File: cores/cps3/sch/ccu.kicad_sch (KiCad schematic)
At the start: 2 parts, among them J13 DL-2829-CCU

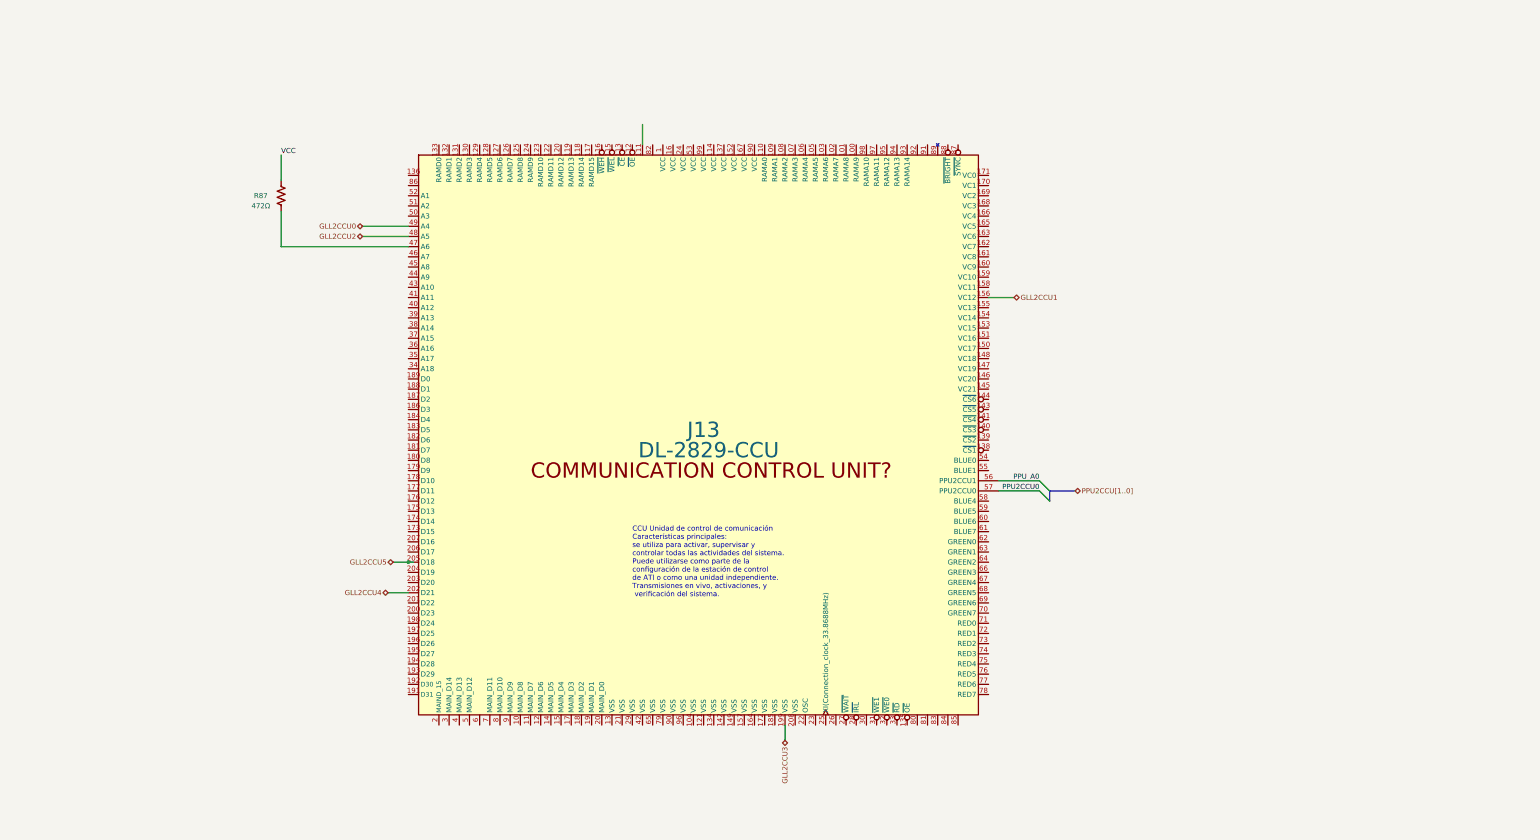
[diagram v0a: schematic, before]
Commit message: wip_ccu_gll2_cassette
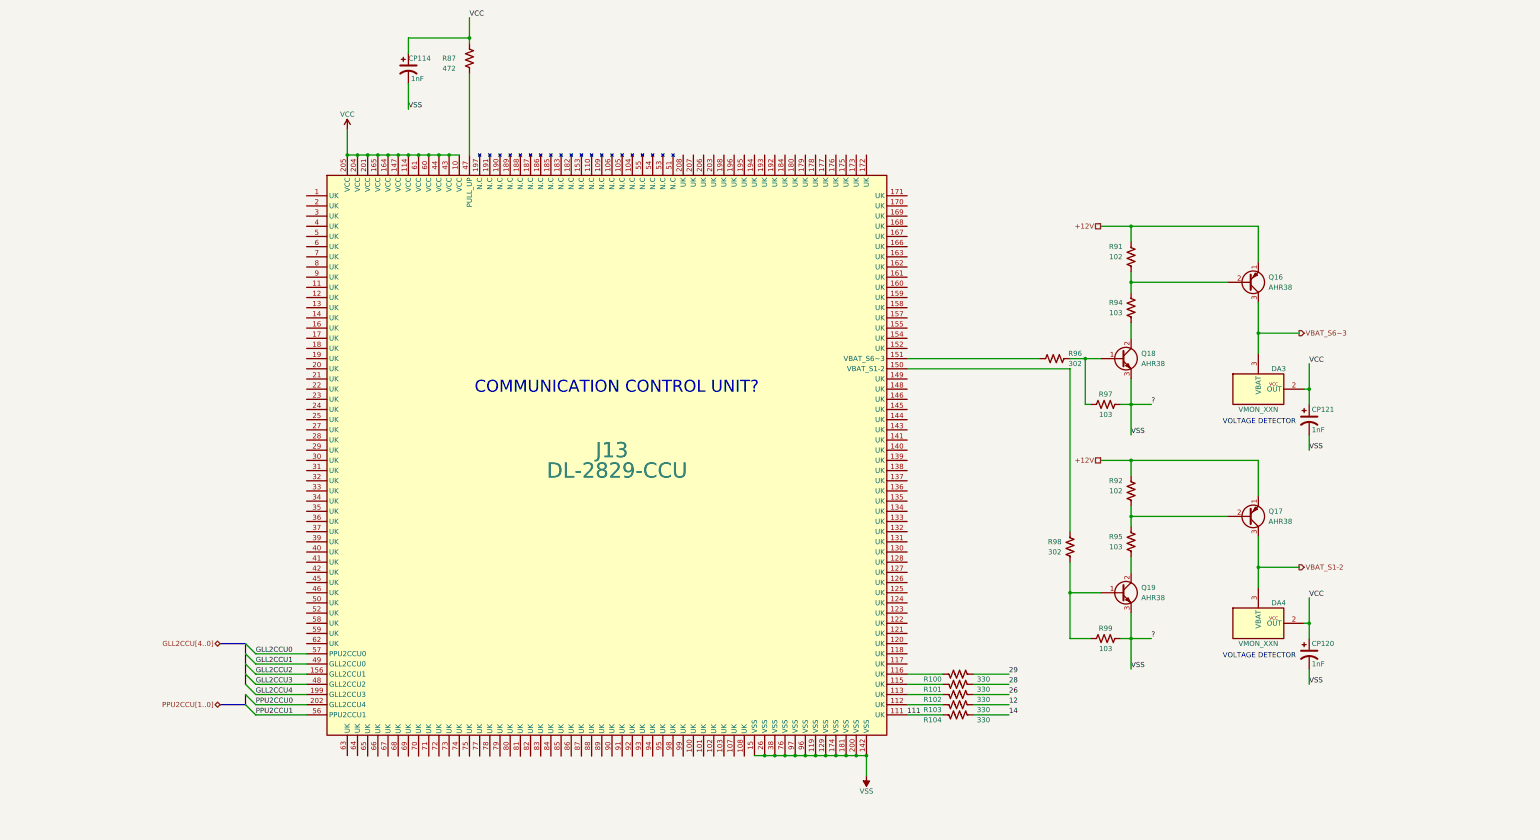
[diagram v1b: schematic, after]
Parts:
- added CP114, CP120, CP121: 1nF, symbol Device:C_Polarized_US
- added DA3, DA4: VMON_XXN, symbol arcade:VMON_XXN
- added Q16, Q17: AHR38, symbol Device:Q_PNP_EBC
- added Q18, Q19: AHR38, symbol Device:Q_NPN_BCE
- added R100, R101, R102, R103, R104: 330, symbol Device:R_US
- added R91, R92: 102, symbol Device:R_US
- added R94, R95, R97, R99: 103, symbol Device:R_US
- added R96, R98: 302, symbol Device:R_US
- R87: value 472Ω -> 472
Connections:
- net GLL2CCU5 is gone; now on net VCC: J13.205 (VCC)
- net GLL2CCU0: now also J13.57 (PPU2CCU0); no longer J13.49 (A4)
- net GLL2CCU1: now also J13.49 (GLL2CCU0); no longer J13.156 (VC12)
- net GLL2CCU2: now also J13.156 (GLL2CCU1); no longer J13.48 (A5)
- net GLL2CCU3: now also J13.48 (GLL2CCU2); no longer J13.199 (VSS)
- net GLL2CCU4: now also J13.199 (GLL2CCU3); no longer J13.202 (D21)
- net PPU2CCU0: now also J13.202 (GLL2CCU4); no longer J13.57 (PPU2CCU0)
- net VCC: now also J13.10 (VCC), J13.114 (VCC), J13.147 (VCC), J13.164 (VCC), J13.165 (VCC), J13.201 (VCC), J13.204 (VCC), J13.43 (VCC), J13.44 (VCC), J13.60 (VCC), J13.61 (VCC), CP114.1, CP120.1, CP121.1, DA3.2 (OUT), DA4.2 (OUT)
- net 111: now reaches J13.111 (UK)
- net 111: now also R104.1
- net at J13.112 (UK): now also R103.1
- net at J13.113 (UK): now also R102.1
- net at J13.115 (UK): now also R101.1
- net at J13.116 (UK): now also R100.1
- net VSS: now reaches J13.119 (VSS)
- net VSS: now also J13.129 (VSS), J13.142 (VSS), J13.15 (VSS), J13.174 (VSS), J13.181 (VSS), J13.200 (VSS), J13.26 (VSS), J13.38 (VSS), J13.76 (VSS), J13.96 (VSS), J13.97 (VSS), CP114.2, CP120.2, CP121.2, DA3.1 (VSS), DA4.1 (VSS), Q18.3 (E), Q19.3 (E), R97.2, R99.2
- net at J13.150 (VBAT_S1-2): now also R98.2
- net at J13.151 (VBAT_S6~3): now also R96.1
- net PPU_A0 renamed PPU2CCU1
- new net: Q18.1 (B), R96.2, R97.1
- new net: Q19.1 (B), R98.1, R99.1
- new net: Q19.2 (C), R95.2
- new net: Q18.2 (C), R94.2
- new net: Q16.2 (B), R91.1, R94.1
- new net: Q17.2 (B), R92.1, R95.1
- new net +12V: Q16.1 (E), Q17.1 (E), R91.2, R92.2
- new net 12: R103.2
- new net 14: R104.2
- new net 26: R102.2
- new net 28: R101.2
- new net 29: R100.2
- new net VBAT_S1-2: DA4.3 (VBAT), Q17.3 (C)
- new net VBAT_S6~3: DA3.3 (VBAT), Q16.3 (C)
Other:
- note added: "COMMUNICATION CONTROL UNIT?"
- note added: "VOLTAGE DETECTOR"
- note removed: "CCU Unidad de control de comunicación Características principales: se utiliza para activar, supervisar y controlar todas las actividades del sistema. Puede utilizarse como parte de la conﬁguración de la estación de control de ATI o como una unidad independiente. Transmisiones en vivo, activaciones, y veriﬁcación del sistema."
- moved on the sheet: R87

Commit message: wip_ccu_cassette
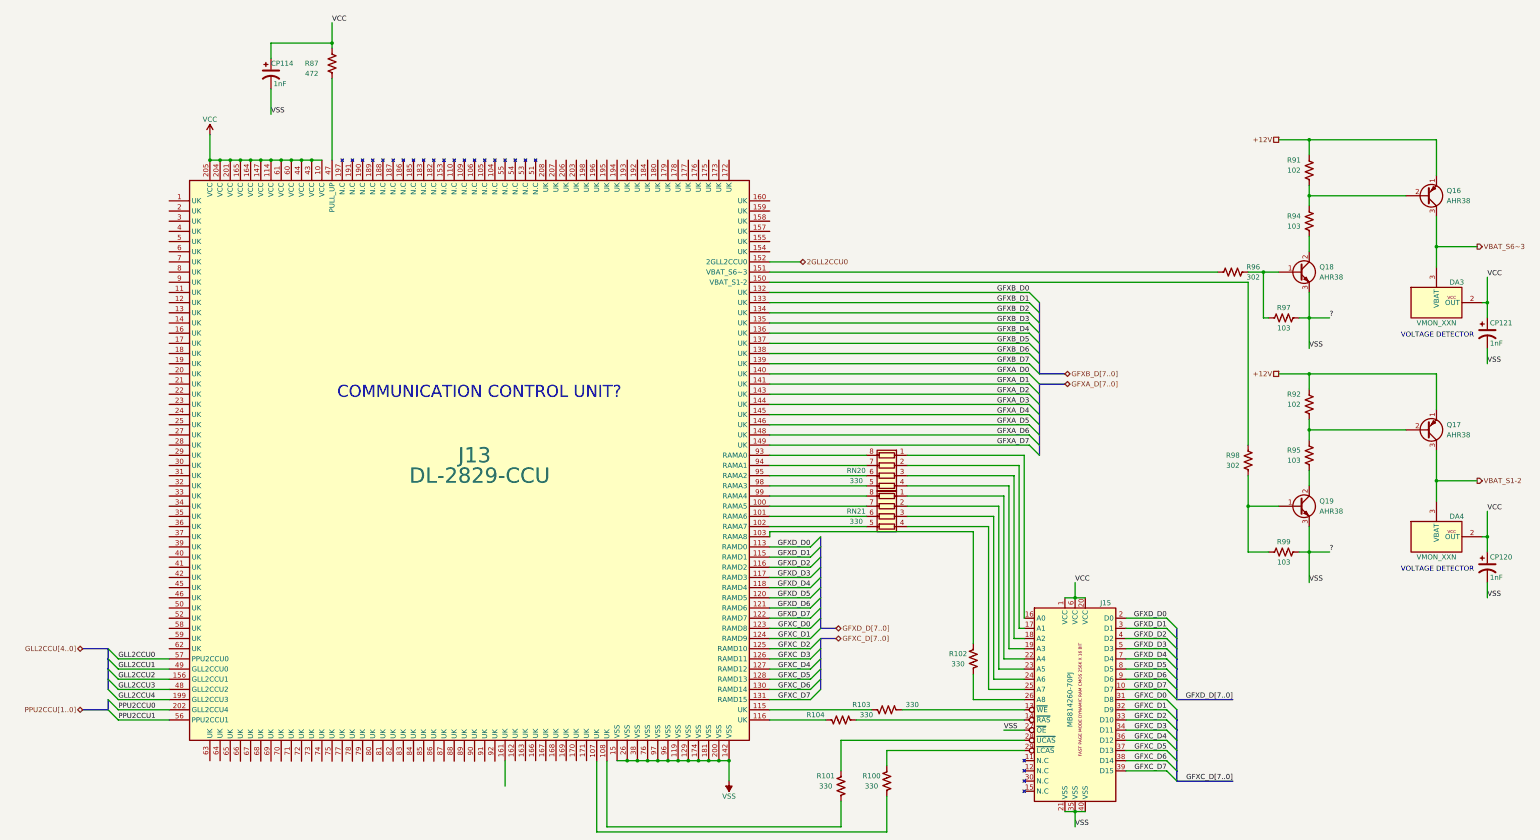
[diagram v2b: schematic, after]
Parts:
- added J15: MB814260-70PJ, symbol fujitsu:MB814260-70PJ
- added RN20, RN21: 330, symbol Device:R_Pack04
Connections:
- net 28 is gone; now on an unnamed net: R101.2
- net 29 is gone; now on an unnamed net: R100.2
- net VCC: now also J15.1 (VCC), J15.20 (VCC), J15.6 (VCC)
- net VSS: now also J15.21 (VSS), J15.27 (~{OE}), J15.35 (VSS), J15.40 (VSS)
- net at R102.1: now also J13.103 (RAMA8); no longer J13.113 (UK)
- net at R100.1: now also J15.29 (~{LCAS}); no longer J13.116 (UK)
- net at J13.100 (RAMA5): now also RN21.7 (R2.2)
- net at J13.101 (RAMA6): now also RN21.6 (R3.2)
- net at J13.102 (RAMA7): now also RN21.5 (R4.2)
- net at R103.1: now also J13.115 (UK); no longer J13.112 (UK)
- net at R101.1: now also J15.28 (~{UCAS}); no longer J13.115 (UK)
- net GFXD_D3: now reaches J13.117 (RAMD3)
- net GFXD_D3: now also J15.5 (D3)
- net GFXD_D4: now reaches J13.118 (RAMD4)
- net GFXD_D4: now also J15.7 (D4)
- net GFXD_D5: now reaches J13.120 (RAMD5)
- net GFXD_D5: now also J15.8 (D5)
- net GFXD_D6: now reaches J13.121 (RAMD6)
- net GFXD_D6: now also J15.9 (D6)
- net GFXD_D7: now reaches J13.122 (RAMD7)
- net GFXD_D7: now also J15.10 (D7)
- net GFXC_D0: now reaches J13.123 (RAMD8)
- net GFXC_D0: now also J15.31 (D8)
- net GFXC_D1: now reaches J13.124 (RAMD9)
- net GFXC_D1: now also J15.32 (D9)
- net GFXC_D2: now reaches J13.125 (RAMD10)
- net GFXC_D2: now also J15.33 (D10)
- net GFXC_D3: now reaches J13.126 (RAMD11)
- net GFXC_D3: now also J15.34 (D11)
- net GFXC_D4: now reaches J13.127 (RAMD12)
- net GFXC_D4: now also J15.36 (D12)
- net GFXC_D5: now reaches J13.128 (RAMD13)
- net GFXC_D5: now also J15.37 (D13)
- net GFXC_D6: now reaches J13.130 (RAMD14)
- net GFXC_D6: now also J15.38 (D14)
- net GFXC_D7: now reaches J13.131 (RAMD15)
- net GFXC_D7: now also J15.39 (D15)
- net GFXB_D0: now reaches J13.132 (UK)
- net GFXB_D1: now reaches J13.133 (UK)
- net GFXB_D2: now reaches J13.134 (UK)
- net GFXB_D3: now reaches J13.135 (UK)
- net GFXB_D4: now reaches J13.136 (UK)
- net GFXB_D5: now reaches J13.137 (UK)
- net GFXB_D6: now reaches J13.138 (UK)
- net GFXB_D7: now reaches J13.139 (UK)
- net GFXA_D0: now reaches J13.140 (UK)
- net GFXA_D1: now reaches J13.141 (UK)
- net GFXA_D2: now reaches J13.143 (UK)
- net GFXA_D3: now reaches J13.144 (UK)
- net GFXA_D4: now reaches J13.145 (UK)
- net GFXA_D5: now reaches J13.146 (UK)
- net GFXA_D6: now reaches J13.148 (UK)
- net GFXA_D7: now reaches J13.149 (UK)
- net 2GLL2CCU0: now reaches J13.152 (2GLL2CCU0)
- net at J13.93 (RAMA0): now also RN20.8 (R1.2)
- net at J13.94 (RAMA1): now also RN20.7 (R2.2)
- net at J13.95 (RAMA2): now also RN20.6 (R3.2)
- net at J13.98 (RAMA3): now also RN20.5 (R4.2)
- net at J13.99 (RAMA4): now also RN21.8 (R1.2)
- net 111: no longer names the net of R104.1
- net 111: now also J13.116 (UK); no longer J13.111 (UK)
- net 12: no longer names the net of R103.2
- net 12: now also J15.13 (~{WE})
- net 14: no longer names the net of R104.2
- net 14: now also J15.14 (~{RAS})
- net 26: no longer names the net of R102.2
- net 26: now also J15.26 (A8)
- new net: J15.16 (A0), RN20.1 (R1.1)
- new net: J15.17 (A1), RN20.2 (R2.1)
- new net: J15.18 (A2), RN20.3 (R3.1)
- new net: J15.19 (A3), RN20.4 (R4.1)
- new net: J15.22 (A4), RN21.1 (R1.1)
- new net: J15.23 (A5), RN21.2 (R2.1)
- new net: J15.24 (A6), RN21.3 (R3.1)
- new net: J15.25 (A7), RN21.4 (R4.1)
- new net GFXD_D0: J13.113 (RAMD0), J15.2 (D0)
- new net GFXD_D1: J13.115 (UK), J15.3 (D1)
- new net GFXD_D2: J13.116 (UK), J15.4 (D2)
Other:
- moved on the sheet: CP114, CP120, CP121, DA3, DA4, J13, Q16, Q17, Q18, Q19, R100, R101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
